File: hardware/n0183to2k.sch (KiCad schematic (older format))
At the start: 41 parts, among them J1 NMEA0183 (wind), J2 Conn_01x06_Male, J3 Conn_01x05_Male, J4 RJ45, J5 RJ45, J6 Conn_02x03_Odd_Even, Q1 BSS123, Q2 DMG2307L, Q3 BSS123, U1 PIC18F27Q84_ISS, U2 TLE9250VSJXUMA1, U3 mic5504-3.3, U4 LDL1117S50, Y1 10Mhz

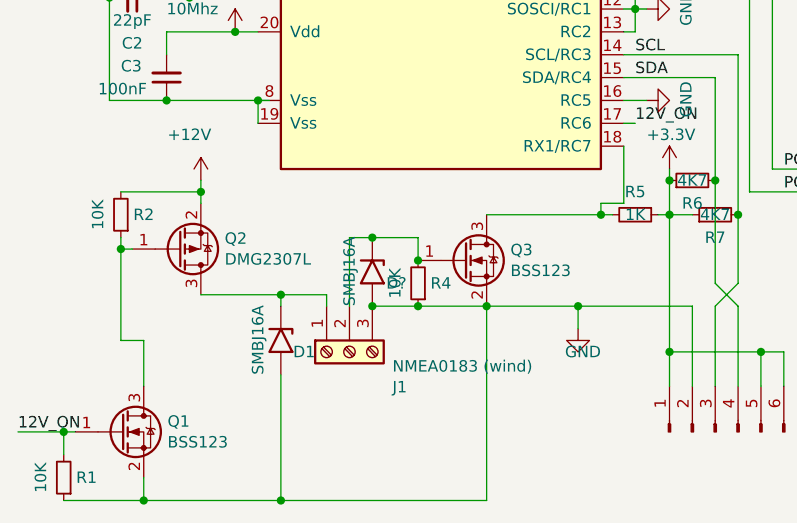
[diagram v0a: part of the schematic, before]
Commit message: Annotate
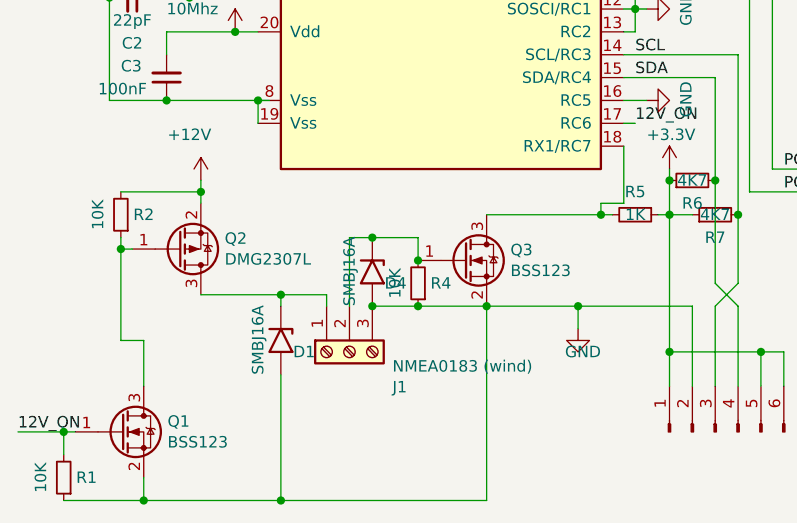
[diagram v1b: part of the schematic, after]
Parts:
- gave numbers to parts that had none: 1
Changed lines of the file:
@@
 $EndComp
 $Comp
-L Diode:1.5KExxA D?
+L Diode:1.5KExxA D4
 U 1 1 622C1983
 P 2450 5900
-F 0 "D?" V 2500 6050 50  0000 R CNN
+F 0 "D4" V 2500 6050 50  0000 R CNN
 F 1 "SMBJ16A" H 2600 5800 50  0000 R CNN
 F 2 "Diode_SMD:D_SMB_Handsoldering" H 2450 5700 50  0001 C CNN
